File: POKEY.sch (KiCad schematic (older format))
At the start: 0 parts

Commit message: PIA and POKEY
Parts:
- added C69, C70: 100nF, Atari:C_Axial_L5.1mm_D2.5mm_P12.50mm_Horizontal, symbol Device:C
- added C75, C76, C77, C78: 1nF, Atari:C_Axial_L5.1mm_D2.5mm_P12.50mm_Horizontal, symbol Device:C
- added D5: 1N4148, Diode_THT:D_DO-35_SOD27_P12.70mm_Horizontal, symbol Diode:1N4148
- added R128, R129, R130, R131, R90: 100, Atari:R_Axial_DIN0207_L3.6mm_D2.2mm_P10.16mm_Horizontal, symbol Device:R
- added R137: 270, Atari:R_Axial_DIN0207_L3.6mm_D2.2mm_P10.16mm_Horizontal, symbol Device:R
- added R138, R139, R140, R141, R142, R143, R144, R145, R146, R147, R148, R149, R150, R151, R152, R153: 220, Atari:R_Axial_DIN0207_L3.6mm_D2.2mm_P10.16mm_Horizontal, symbol Device:R
- added R74, R75: 3k, Atari:R_Axial_DIN0207_L3.6mm_D2.2mm_P10.16mm_Horizontal, symbol Device:R
- added R80: 1k, Atari:R_Axial_DIN0207_L3.6mm_D2.2mm_P10.16mm_Horizontal, symbol Device:R
- added R81, R82, R83, R84: 4k7, Atari:R_Axial_DIN0207_L3.6mm_D2.2mm_P10.16mm_Horizontal, symbol Device:R
- added R89, R96: 47k, Atari:R_Axial_DIN0207_L3.6mm_D2.2mm_P10.16mm_Horizontal, symbol Device:R
- added U22: POKEY, Package_DIP:DIP-40_W15.24mm_Socket, symbol Atari:POKEY
- added U24, U25: CD4051B, Package_DIP:DIP-18_W7.62mm_Socket, symbol Analog_Switch:CD4051B
- added W1: 0, Atari:R_Axial_DIN0207_L3.6mm_D2.2mm_P10.16mm_Horizontal, symbol Device:R
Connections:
- new net: R75.1, U22.10 (P4), W1.1
- new net: D5.2 (A), R137.2, R96.1, U22.16 (~KR2)
- new net: R130.2, R83.2, U22.24 (SID)
- new net: R89.1, U22.25 (~KR1), U24.3 (X)
- new net: R129.2, R82.2, U22.26 (BCLK)
- new net: R128.2, R81.2, U22.27 (ACLK)
- new net: R131.2, R84.2, U22.28 (SOD)
- new net: R74.2, U22.31 (CS1)
- new net: R150.2, U24.1 (X4)
- new net: R149.2, U24.12 (X3)
- new net: R146.2, U24.13 (X0)
- new net: R147.2, U24.14 (X1)
- new net: R148.2, U24.15 (X2)
- new net: R152.2, U24.2 (X6)
- new net: R153.2, U24.4 (X7)
- new net: R151.2, U24.5 (X5)
- new net: R141.2, U25.1 (X4)
- new net: R142.2, U25.12 (X3)
- new net: R145.2, U25.13 (X0)
- new net: R144.2, U25.14 (X1)
- new net: R143.2, U25.15 (X2)
- new net: C70.1, U25.16 (VDD)
- new net: R139.2, U25.2 (X6)
- new net: R90.1, U25.3 (X)
- new net: R138.2, U25.4 (X7)
- new net: R140.2, U25.5 (X5)
- new net +5P: R80.2
- new net +5VA: C69.1, D5.1 (K), R74.1, R75.2, R81.1, R82.1, R83.1, R84.1, R89.2, R96.2, U24.16 (VDD)
- new net A0: U22.36 (A0)
- new net A1: U22.35 (A1)
- new net A2: U22.34 (A2)
- new net A3: U22.33 (A3)
- new net AUDIO: R80.1, U22.37 (AUDIO)
- new net BSC: R137.1
- new net CLK_IN: C76.1, R129.1
- new net CLK_OUT: C75.1, R128.1
- new net D0: U22.38 (D0)
- new net D1: U22.39 (D1)
- new net D2: U22.40 (D2)
- new net D3: U22.2 (D3)
- new net D4: U22.3 (D4)
- new net D5: U22.4 (D5)
- new net D6: U22.5 (D6)
- new net D7: U22.6 (D7)
- new net DATA_IN: C77.1, R130.1
- new net DATA_OUT: C78.1, R131.1
- new net GND: C69.2, C70.2, C75.2, C76.2, C77.2, C78.2, R90.2, U22.11 (P5), U22.8 (P6), U22.9 (P7), U24.6 (INH), U24.7 (VEE), U24.8 (VSS), U25.6 (INH), U25.7 (VEE), U25.8 (VSS), W1.2
- new net IN0: R146.1
- new net IN1: R147.1
- new net IN2: R148.1
- new net IN3: R149.1
- new net IN4: R150.1
- new net IN5: R151.1
- new net IN6: R152.1
- new net IN7: R153.1
- new net IRQ: U22.29 (~IRQ)
- new net K0: U22.23 (~K0), U24.9 (C)
- new net K1: U22.22 (~K1), U24.10 (B)
- new net K2: U22.21 (~K2), U24.11 (A)
- new net K3: U22.20 (~K3), U25.11 (A)
- new net K4: U22.19 (~K4), U25.10 (B)
- new net K5: U22.18 (~K5), U25.9 (C)
- new net O2: U22.7 (O2)
- new net OUT0: R145.1
- new net OUT1: R144.1
- new net OUT2: R143.1
- new net OUT3: R142.1
- new net OUT4: R141.1
- new net OUT5: R140.1
- new net OUT6: R139.1
- new net OUT7: R138.1
- new net POKEY: U22.30 (~CS0)
- new net RW: U22.32 (R/~W)

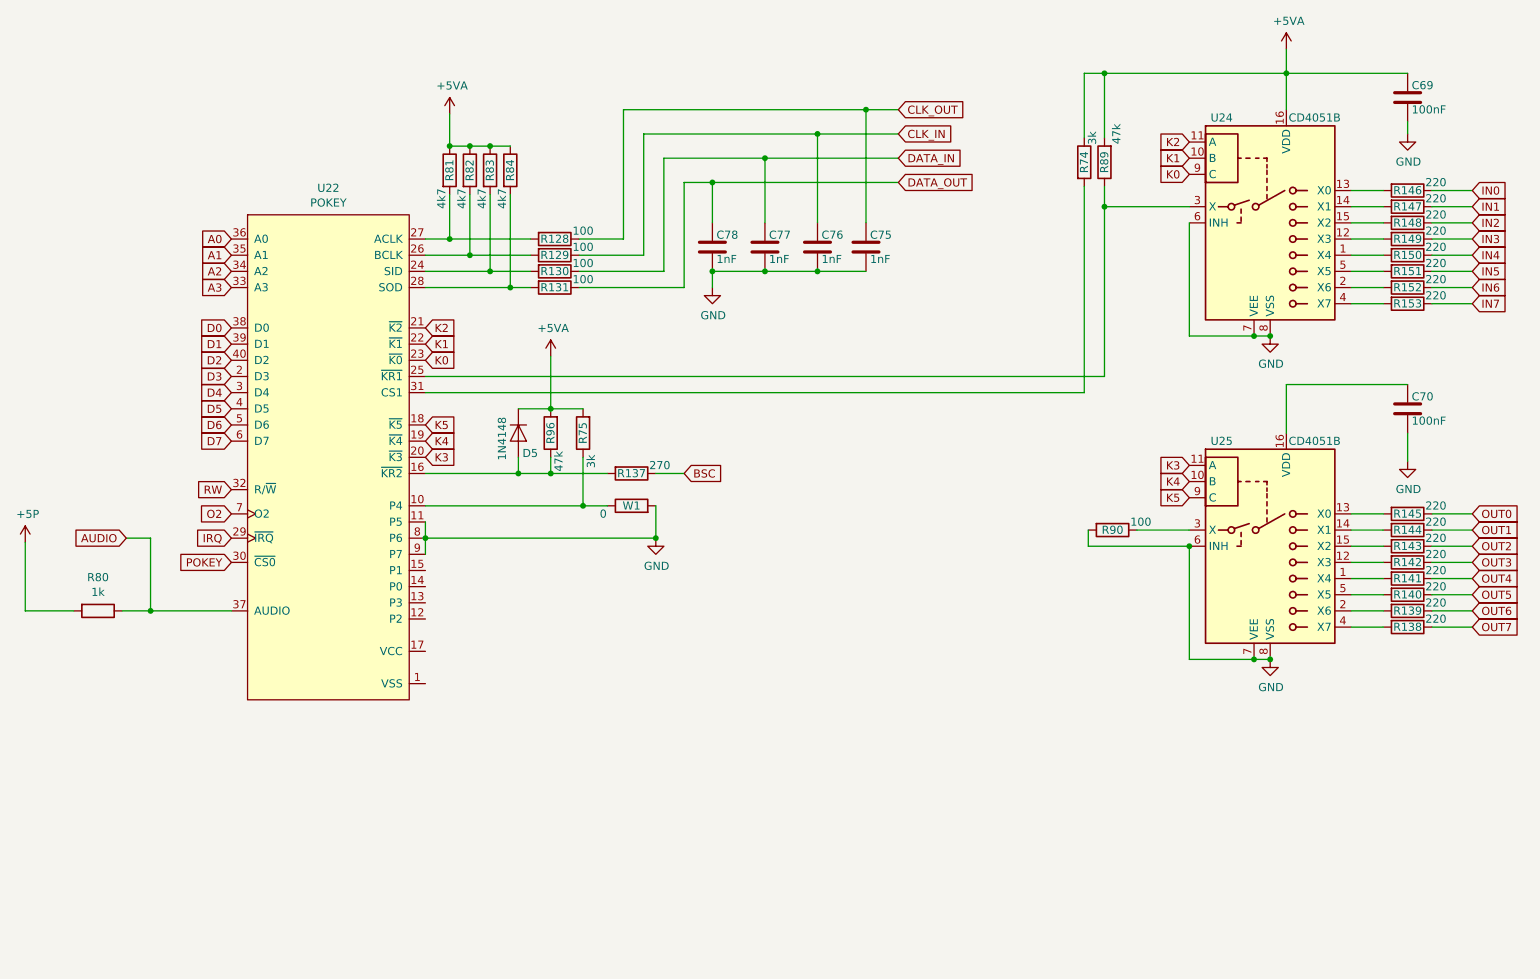
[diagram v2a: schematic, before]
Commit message: Pokey finish
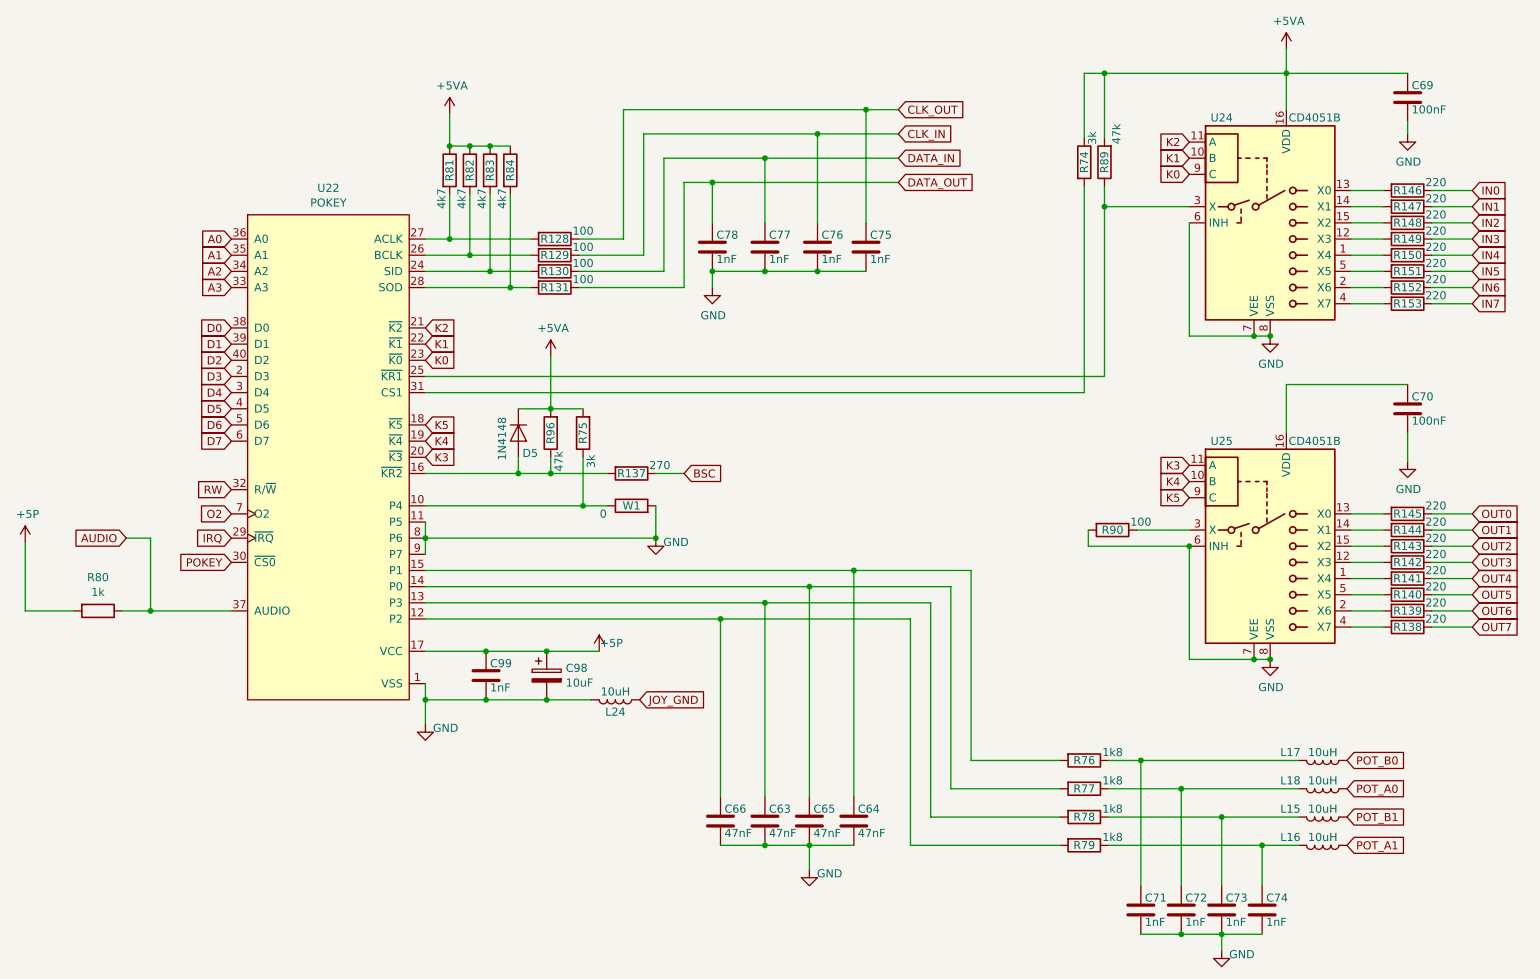
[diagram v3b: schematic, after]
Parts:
- added C63, C64, C65, C66: 47nF, Atari:C_Axial_L5.1mm_D2.5mm_P12.50mm_Horizontal, symbol Device:C
- added C71, C72, C73, C74, C99: 1nF, Atari:C_Axial_L5.1mm_D2.5mm_P12.50mm_Horizontal, symbol Device:C
- added C98: 10uF, Capacitor_THT:CP_Radial_Tantal_D5.0mm_P2.50mm, symbol Device:CP
- added L15, L16, L17, L18, L24: 10uH, Atari:L_Axial_L7.0mm_D3.3mm_P12.50mm_Horizontal_Fastron_MICC, symbol Device:L
- added R76, R77, R78, R79: 1k8, Atari:R_Axial_DIN0207_L3.6mm_D2.2mm_P10.16mm_Horizontal, symbol Device:R
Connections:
- net +5P: now also U22.17 (VCC), C98.1, C99.1
- net GND: now also U22.1 (VSS), C63.2, C64.2, C65.2, C66.2, C71.2, C72.2, C73.2, C74.2, C98.2, C99.2, L24.2
- net at U22.12 (P2): now also C66.1, R79.2
- net at U22.13 (P3): now also C63.1, R78.2
- net at U22.14 (P0): now also C65.1, R77.2
- net at U22.15 (P1): now also C64.1, R76.2
- new net: C71.1, L17.2, R76.1
- new net: C72.1, L18.2, R77.1
- new net: C73.1, L15.2, R78.1
- new net: C74.1, L16.2, R79.1
- new net JOY_GND: L24.1
- new net POT_A0: L18.1
- new net POT_A1: L16.1
- new net POT_B0: L17.1
- new net POT_B1: L15.1
